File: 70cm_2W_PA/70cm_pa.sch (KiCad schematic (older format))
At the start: 48 parts, among them J3 Conn_01x02, U1 M68710L, U2 MIC5205YM5, U3 SN74LV1T08

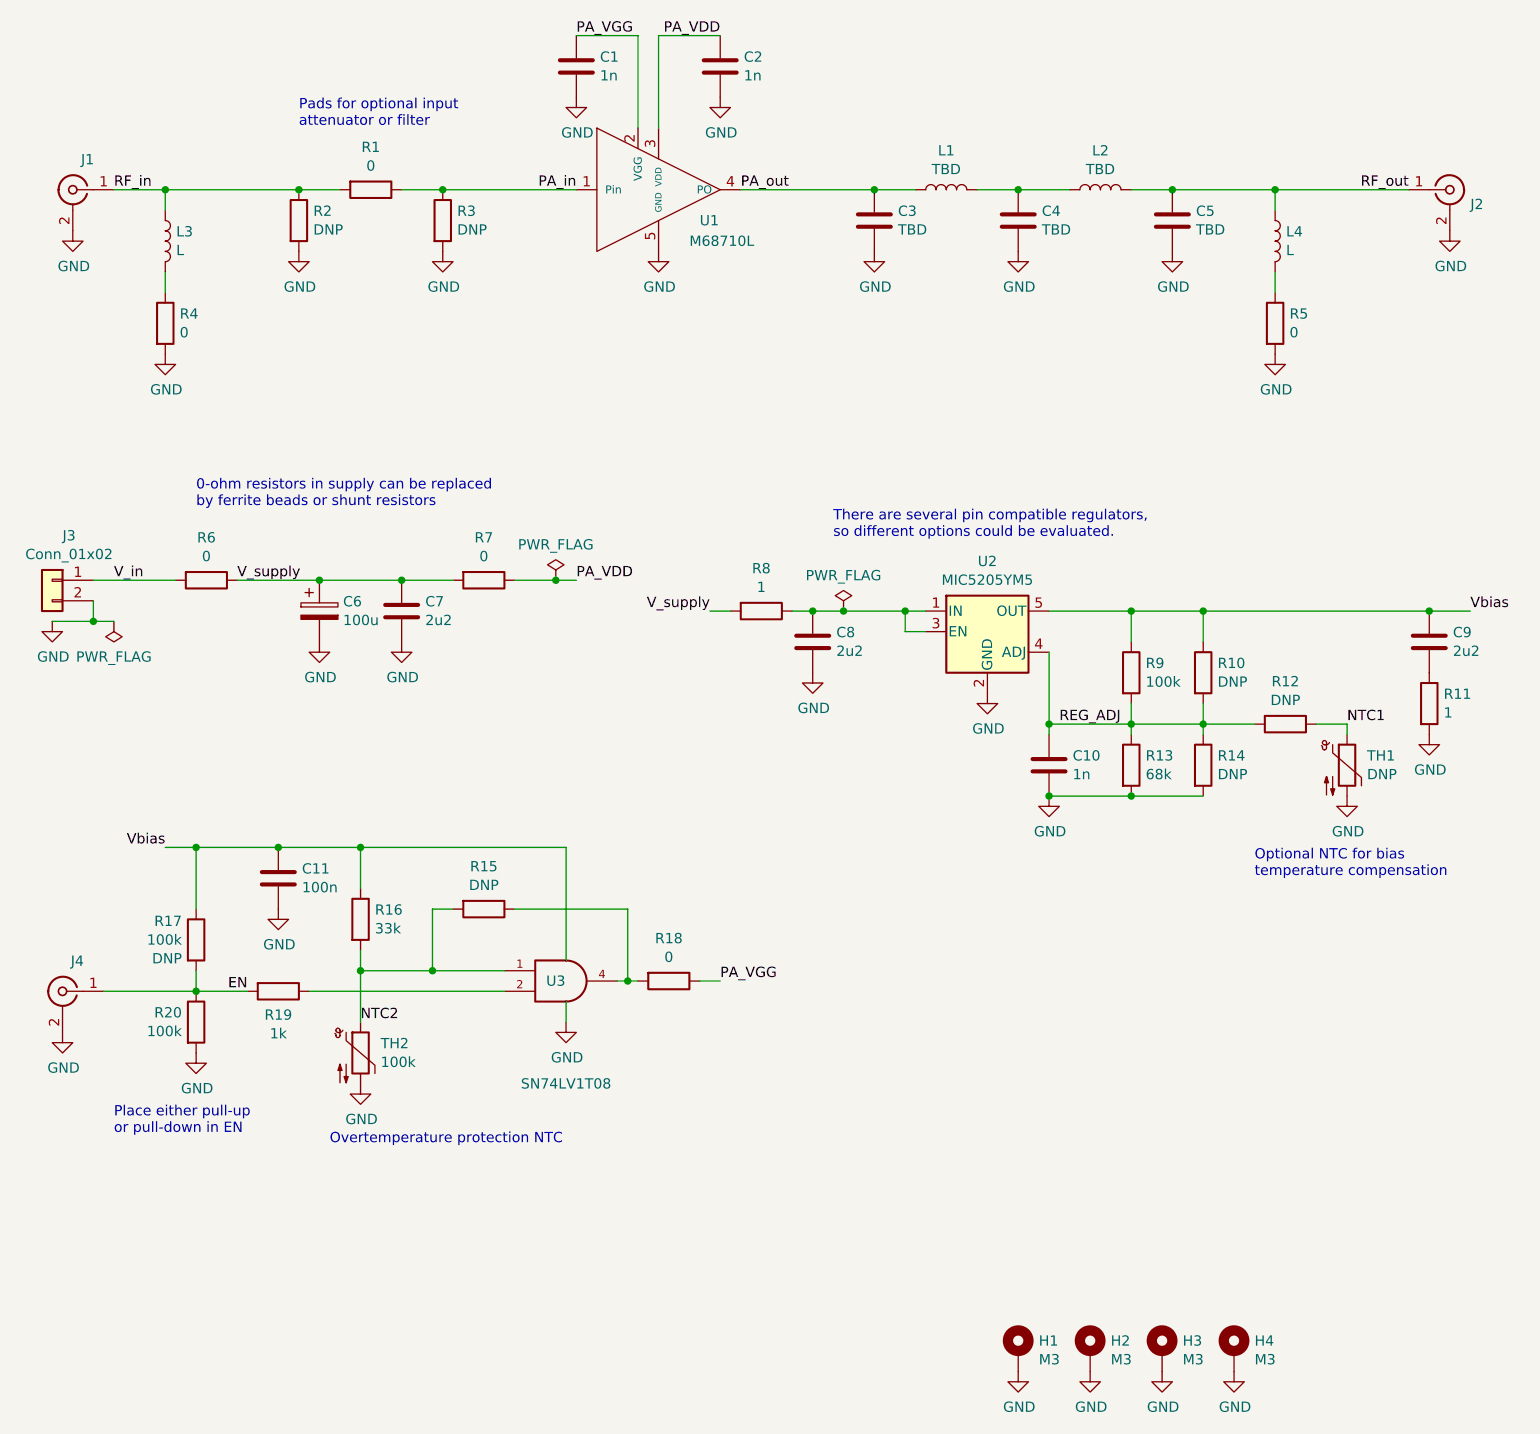
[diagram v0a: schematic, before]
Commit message: M68710L: everything is connected again
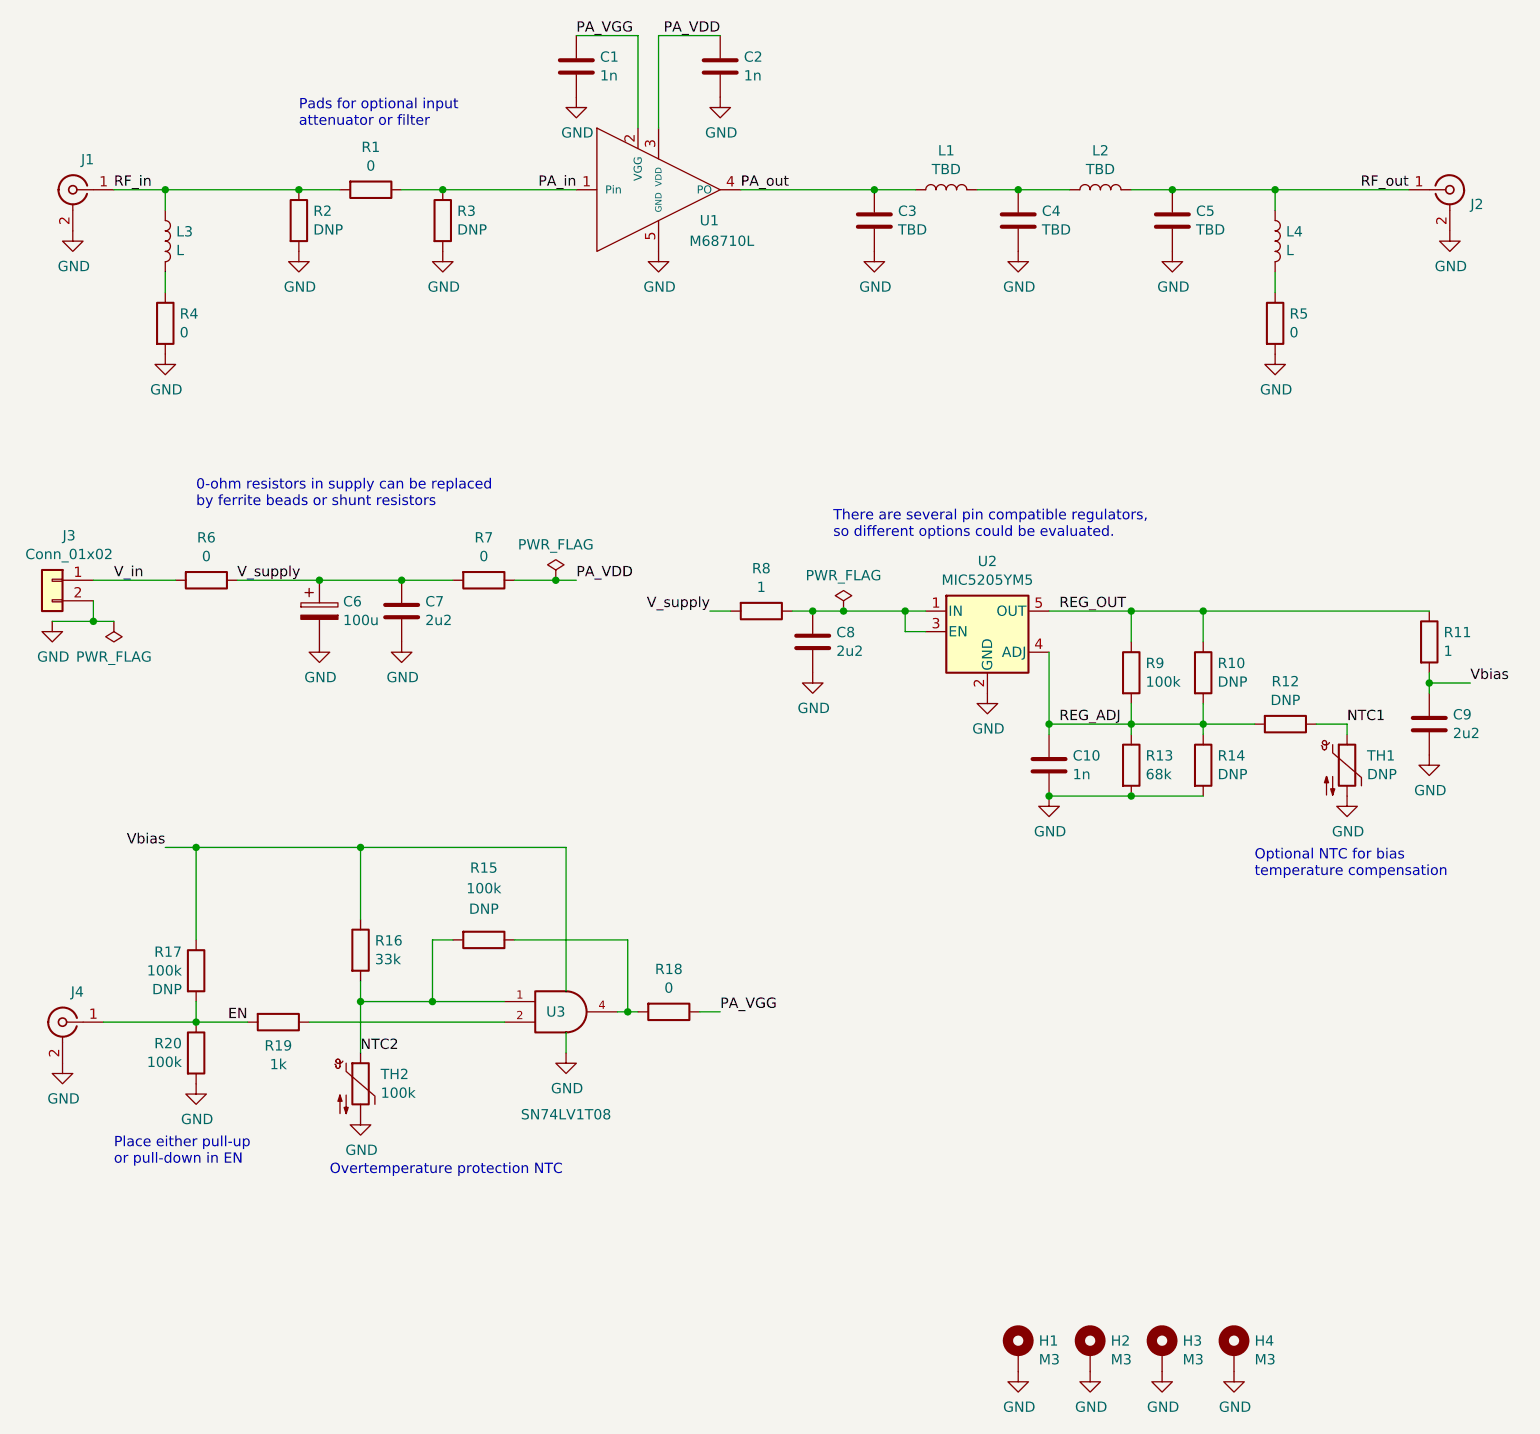
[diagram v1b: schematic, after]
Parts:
- removed C11: 100n, Capacitor_SMD:C_0805_2012Metric, symbol Device:C
- R15: value ~ -> 100k
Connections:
- net GND: now also C9.2; no longer R11.2
- net VCC: now also R11.2; no longer R10.1, R9.1, U2.5 (OUT)
- net REG_OUT: now reaches R11.1
- net REG_OUT: now also R10.1, R9.1, U2.5 (OUT); no longer C9.2
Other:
- moved on the sheet: C9, J4, R11, R15, R16, R17, R18, R19, R20, TH2, U3
